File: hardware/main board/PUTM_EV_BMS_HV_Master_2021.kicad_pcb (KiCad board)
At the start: 4 copper layers, 60 x 150 mm, 246 parts, among them IC1 MCP1501-10E_SN, IC10 REF193GSZ-REEL, IC11 AP7365-33YRG-13, IC12 UCC12040DVE, IC13 MAX17643ATC+, IC14 RTQ2965GSP-QA, IC15 ISO6763FDWR, IC16 ISO6763FDWR, IC17 UCC12040DVE, IC2 MCP3561T-E_NC, IC3 REF193GSZ-REEL, IC4 MCP3561T-E_NC, IC6 AP7365-33YRG-13, IC7 MCP3562T-E_NC, IC9 REF193GSZ-REEL, J1 USB4145-03-0070-C, J10 M80-5100622, J11 M80-5101422, J14 Conn_01x05, J16 TagConnect, J2 M80-5100442, J3 M80-5100442, J4 M300-MV10345M1, J5 M300-MV10345M1, J6 M80-5100442, J7 M80-5100622, J8 M80-5102022, J9 M300-MV30645M1, K2 6-1419128-4, Q1 2SK3065, Q10 Q_NMOS_GSD, Q11 Q_NMOS_GSD, Q12 2SK3065, Q13 2SK3065, Q14 2SK3065, Q15 2SK3065, Q2 2N7002, Q3 Q_NMOS_GDS, Q4 2N7002, Q5 Q_NMOS_GDS, Q6 Q_NMOS_GDS, Q7 2SK3065, Q8 Q_PMOS_GSD, Q9 2SK3065, T1 HX1188NL, U12 LTC6820IMS, U13 LTC6820IMS, U14 74AUP1G32, U2 STM32G484RETx, U3 MCP2542FDxMF, U4 USBLC6-2SC6, U5 LM1117-3.3, U6 MCP2542FDxMF, U8 74LVC1G86, Y1 20MHz, Y2 32.768kHz

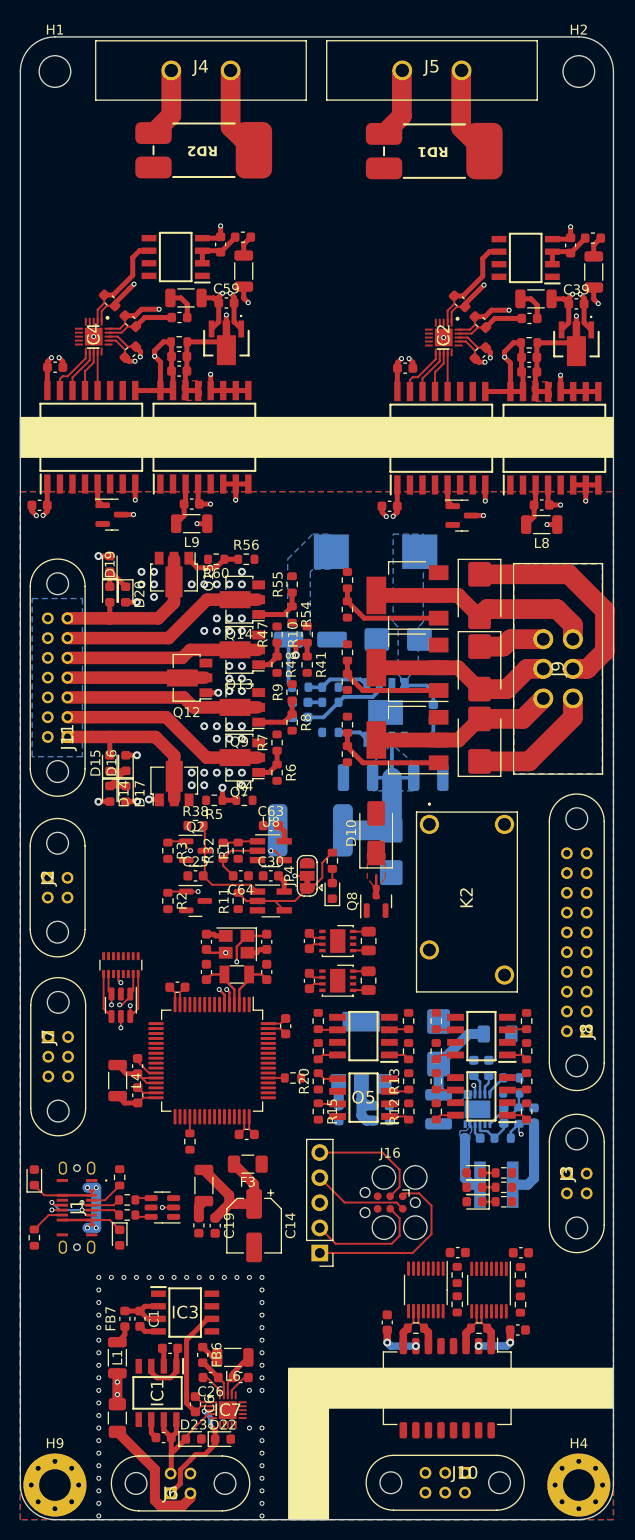
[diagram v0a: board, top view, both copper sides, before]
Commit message: done power plane layout
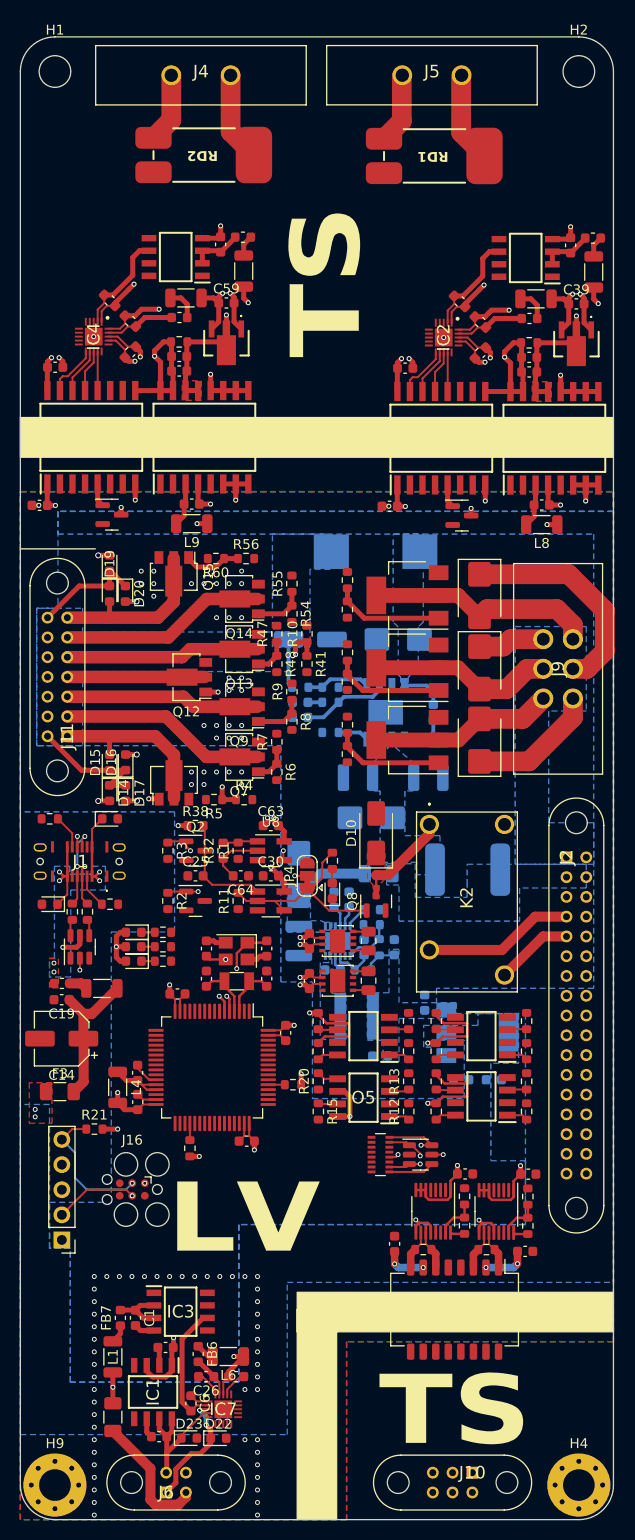
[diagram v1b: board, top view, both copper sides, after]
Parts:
- removed J3: M80-5100442, Samacsys:M80-51004YY
- removed J7: M80-5100622, Samacsys:M80-51006YY
- removed J8: M80-5102022, Samacsys:M80-51020YY
- added C8: 47uF, Capacitor_SMD:C_0603_1608Metric, B.Cu at (143.4, 136.1)
- added R21: 10k, Resistor_SMD:R_0603_1608Metric, F.Cu at (114.5, 143.5)
- C68: value 22uF -> 47uF
- J2: value M80-5100442 -> M80-5103422; footprint Samacsys:M80-51004YY -> Samacsys:M80-51034YY
- moved J2 52.5 mm to (162.2, 116.0)
- moved R19 42.4 mm to (110.0, 112.1), turned to 180 degrees
- moved D7 42.2 mm to (118.5, 123.6)
- moved R69 42.2 mm to (121.4, 126.5)
- moved D5 42.2 mm to (118.5, 126.5)
- moved D6 42.2 mm to (118.5, 125.0)
- moved R71 42.2 mm to (121.4, 125.0)
- moved R72 42.2 mm to (121.4, 123.6)
- moved D21 37.1 mm to (116.1, 112.1), turned to 0 degrees
- moved J1 35.0 mm to (113.0, 116.4), turned to 180 degrees
- moved D1 34.5 mm to (110.0, 120.7), turned to 180 degrees
- moved D8 33.9 mm to (147.5, 146.1), turned to 0 degrees
- moved RN2 32.5 mm to (143.4, 146.1), turned to 0 degrees
- moved R50 31.2 mm to (112.3, 121.5), turned to -90 degrees
- moved R49 29.4 mm to (113.8, 121.5), turned to 90 degrees
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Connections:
- J2 pad 1: GND -> SAFETY_TSMS_IN
- J2 pad 2: AIR_PRE_DETECTION -> VDD
- J2 pad 3: AIR_P_DETECTION -> GND
- J2 pad 4: AIR_M_DETECTION -> AMS_SAFETY_1
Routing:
- net +3V3: track 64.8 -> 113.8 mm, vias 4 -> 28
- net Net-(D3-K): track 18.4 -> 0.00 mm
- net +12V: track 14.5 -> 29.8 mm
- net AMS_SAFETY_1: track 0.00 -> 15.3 mm
- net +5V: track 20.9 -> 8.55 mm, vias 6 -> 5
- net Net-(D10-K): track 1.70 -> 9.77 mm
- net AMS_SAFETY_2: track 0.00 -> 7.89 mm
- net /Safeties and related/AMS_FAULT: track 14.1 -> 21.1 mm
- net Net-(IC13-LX): track 5.85 -> 0.00 mm
- net Net-(U12-ICMP): track 0.00 -> 4.28 mm
- net Net-(U13-ICMP): track 0.00 -> 4.27 mm
- net SWCLK: track 12.2 -> 8.45 mm, vias 0 -> 1
- net VBUS: track 21.5 -> 18.4 mm, vias 4 -> 7
- net GND: track 55.5 -> 58.3 mm, vias 100 -> 96
- net NRST: track 14.0 -> 16.0 mm, vias 0 -> 1
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- added copper zone on B.Cu, net +3V3
- added copper zone on B.Cu, net +5V
- added copper zone on F.Cu, net +5V
- added copper zone on B.Cu, net Net-(D6-K)
- added copper zone on B.Cu, net VBUS
- added copper zone on F.Cu, net VBUS
- added copper zone on B.Cu, net VDD
- removed copper zone on In1.Cu, net +12V
- removed copper zone on B.Cu, net Net-(D2-K)
- removed copper zone on In1.Cu, net SAFETY_TSMS_IN
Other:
- board text added: "LV"
- board text added: "TS"
